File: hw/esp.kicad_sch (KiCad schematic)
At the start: 12 parts, among them SW2 EN, SW3 BOOT, U5 ESP32-S3-WROOM

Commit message: add routing
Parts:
- SW2, SW3: footprint RLK-ElectorMechanicalComponents:TCF2QR -> RLK-ElectorMechanicalComponents:Tactile_switch
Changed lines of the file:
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@@
       (effects (font (size 1.27 1.27)) (justify right))
     )
-    (property "Footprint" "RLK-ElectorMechanicalComponents:TCF2QR" (at 134.62 129.54 0)
+    (property "Footprint" "RLK-ElectorMechanicalComponents:Tactile_switch" (at 134.62 129.54 0)
       (effects (font (size 1.27 1.27)) hide)
     )
@@
       (effects (font (size 1.27 1.27)) (justify right))
     )
-    (property "Footprint" "RLK-ElectorMechanicalComponents:TCF2QR" (at 121.92 129.54 0)
-      (effects (font (size 1.27 1.27)) hide)
-    )
+    (property "Footprint" "RLK-ElectorMechanicalComponents:Tactile_switch" (at 121.92 129.54 0)
+      (effects (font (size 1.27 1.27)) hide)
+    )

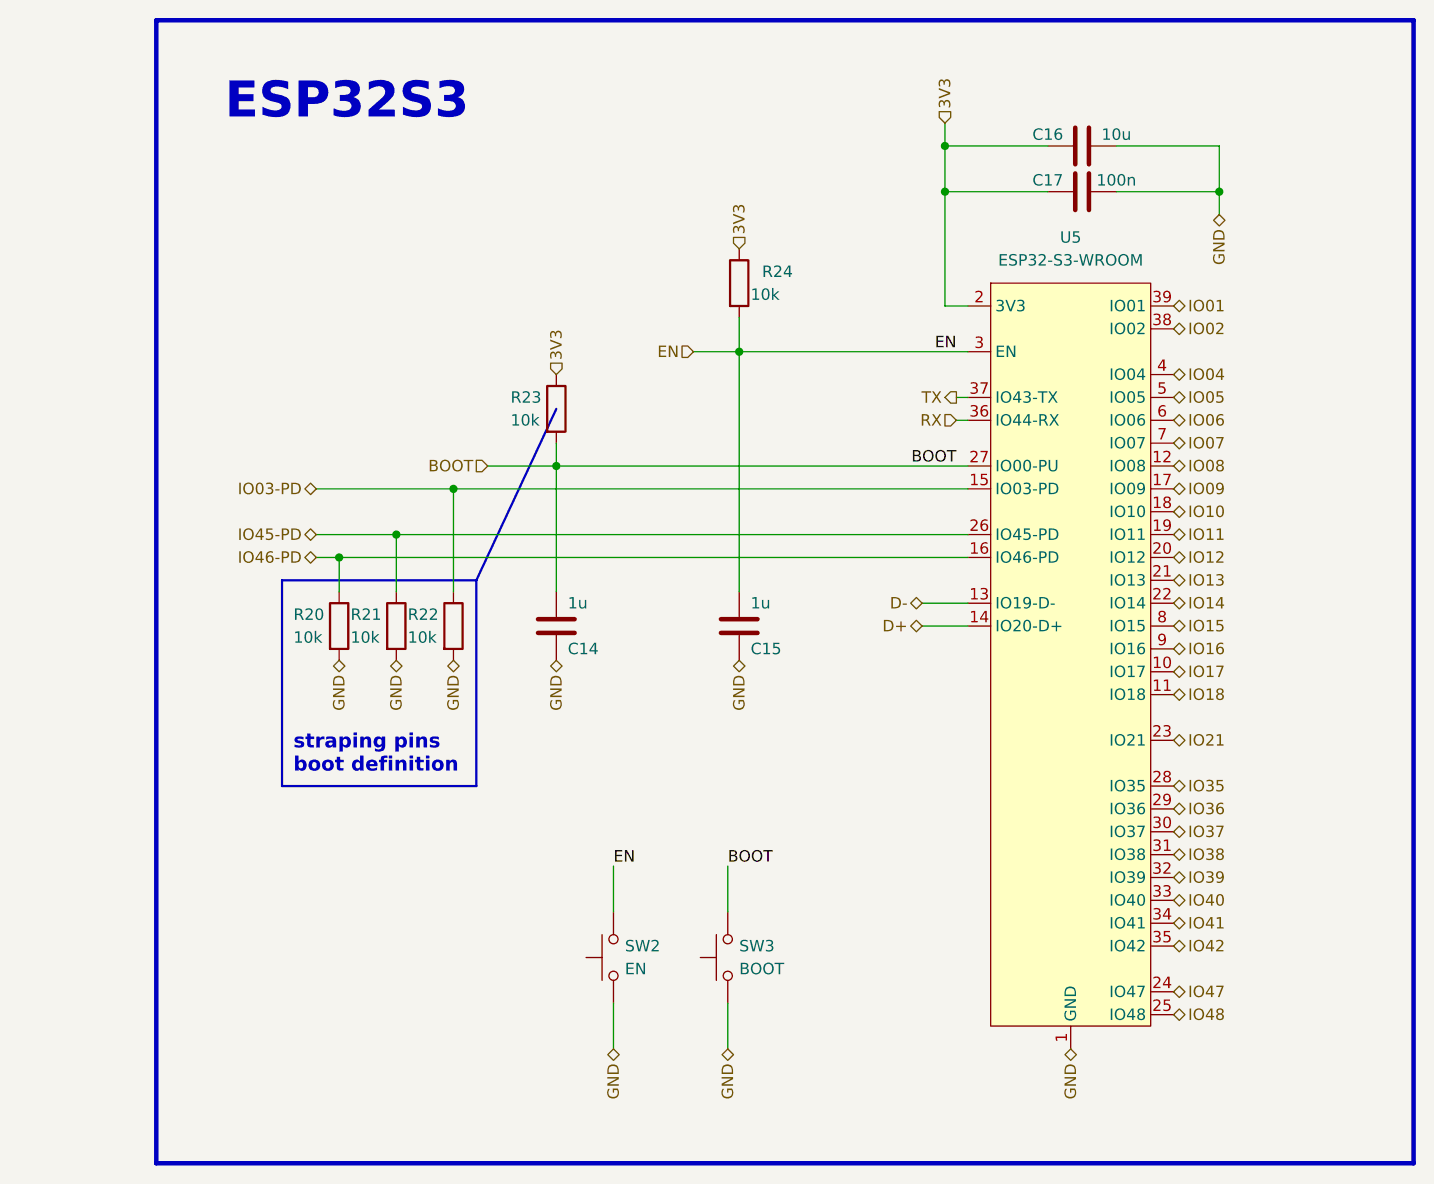
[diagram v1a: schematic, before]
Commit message: Component inspection wip 0
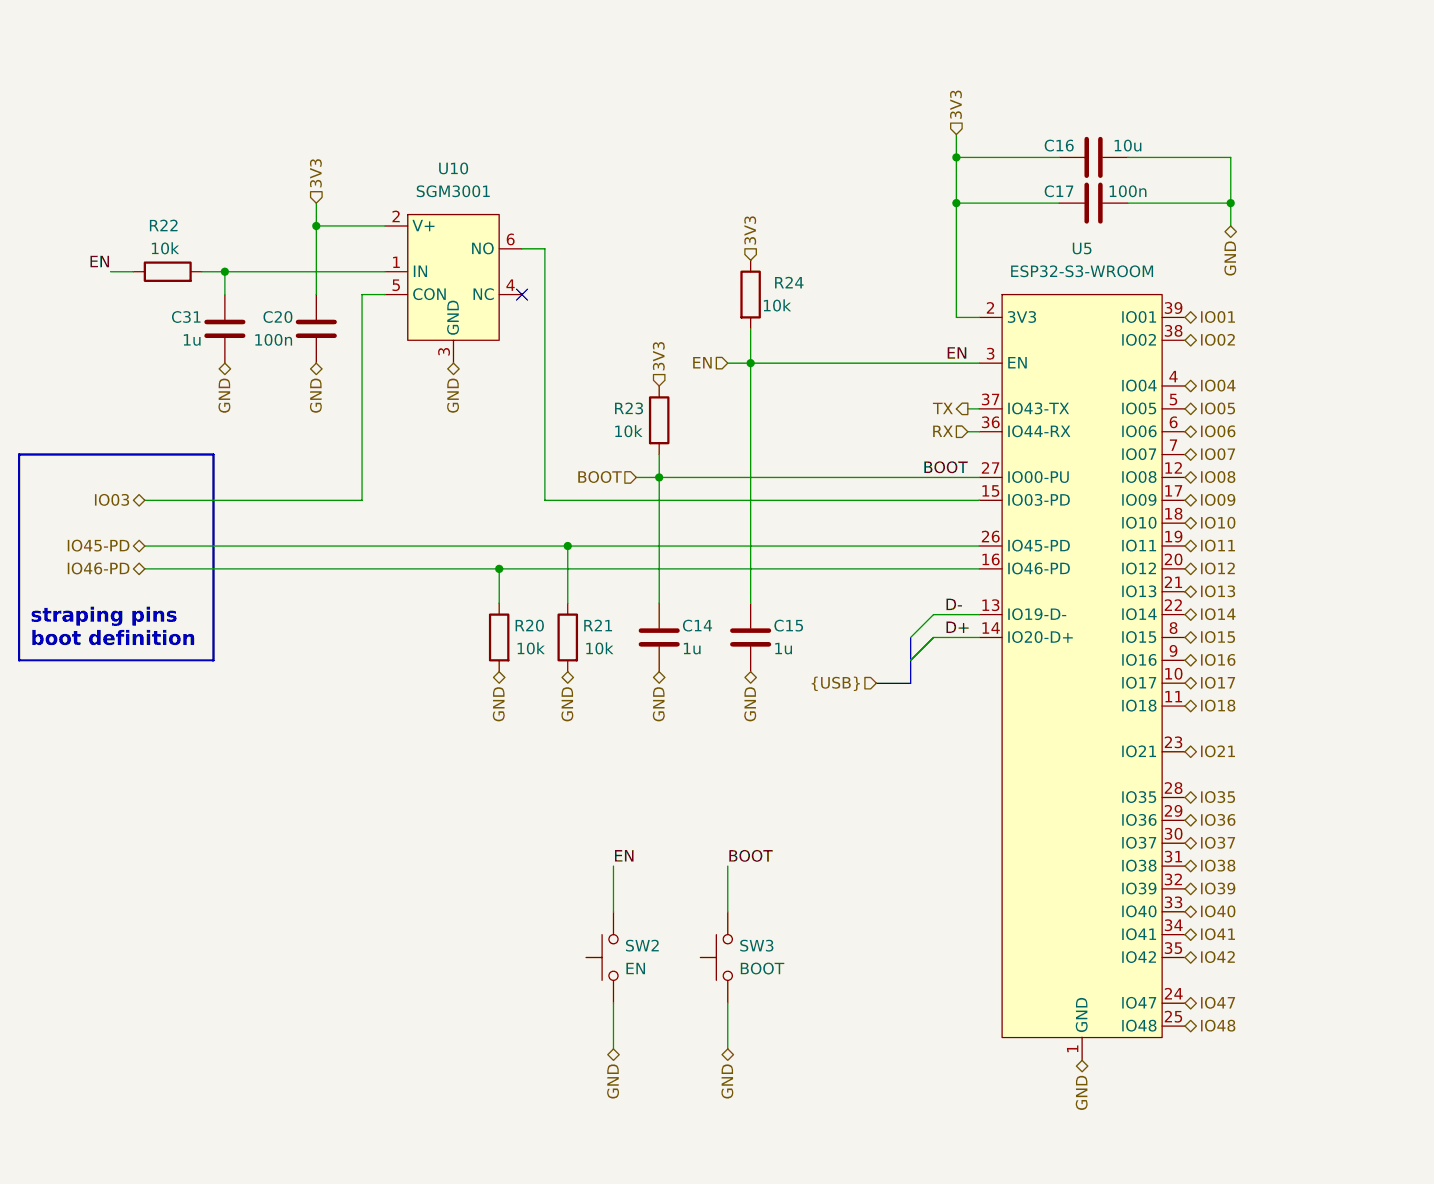
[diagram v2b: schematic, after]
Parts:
- added C20: 100n, Capacitor_SMD:C_0402_1005Metric, symbol Device:C
- added C31: 1u, Capacitor_SMD:C_0402_1005Metric, symbol Device:C
- added U10: SGM3001, Package_TO_SOT_SMD:SOT-363_SC-70-6, symbol RKL-SpecialThings:SGM3001
- C14, C15: Basic/Extended E -> B; LCSC C1518208 -> C52923; info 50V, X5R (potenciálně C52923 což je 25V, X5R ) -> 25V, X5R
- C17: LCSC C307331 -> C1525; info 50V, X7R -> 16V, X7R
- R20, R21, R22, R23, R24: JLCPCB_CORRECTION 0;0;0 -> (none)
- SW2, SW3: footprint RLK-ElectorMechanicalComponents:Tactile_switch -> Button_Switch_SMD:SW_Push_1P1T_NO_Vertical_Wuerth_434133025816; LCSC C240292 -> C127488
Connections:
- net 3V3: now also C20.1, U10.2 (V+)
- net EN: now also R22.1
- net GND: now also C20.2, C31.2, U10.3 (GND); no longer R22.2
- net IO03-PD: no longer names the net of U5.15 (IO03-PD)
- net IO03-PD: now also U10.6 (NO); no longer R22.1
- new net: C31.1, R22.2, U10.1 (IN)
- new net IO03: U10.5 (CON)
- no-connect marks 0 -> 1
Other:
- note removed: "ESP32S3"
- moved on the sheet: C14, C15, C16, C17, R20, R21, R23, R24, U5

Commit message: Inspection of parts complete
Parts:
- U5: LCSC C3013946 -> C2913202
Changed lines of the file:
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@@
       (effects (font (size 1.27 1.27)) hide)
     )
-    (property "LCSC" "C3013946" (at 179.07 43.18 0)
+    (property "LCSC" "C2913202" (at 179.07 43.18 0)
       (effects (font (size 1.27 1.27)) hide)
     )
